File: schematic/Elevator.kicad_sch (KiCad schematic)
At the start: 25 parts, among them M1 Stepper_Motor_bipolar, Q1 Q_NMOS_GDS, Q2 Q_NMOS_GDS, Q3 Q_NMOS_GDS, SW1 SW_Push_LED, SW10 SW_Push_LED, SW11 SW_Push_LED, SW12 SW_Push_LED, SW13 SW_Push_LED, SW14 SW_Push_LED, SW15 SW_Push_LED, SW16 SW_Push_LED, SW2 SW_Push_LED, SW3 SW_Push_LED, SW4 SW_Push_LED, SW5 SW_Push_LED, SW6 SW_Push_LED, SW7 SW_Push_LED, SW8 SW_Push_LED, SW9 SW_Push_LED, U1 Pico, U2 74HC595, U3 74HC595

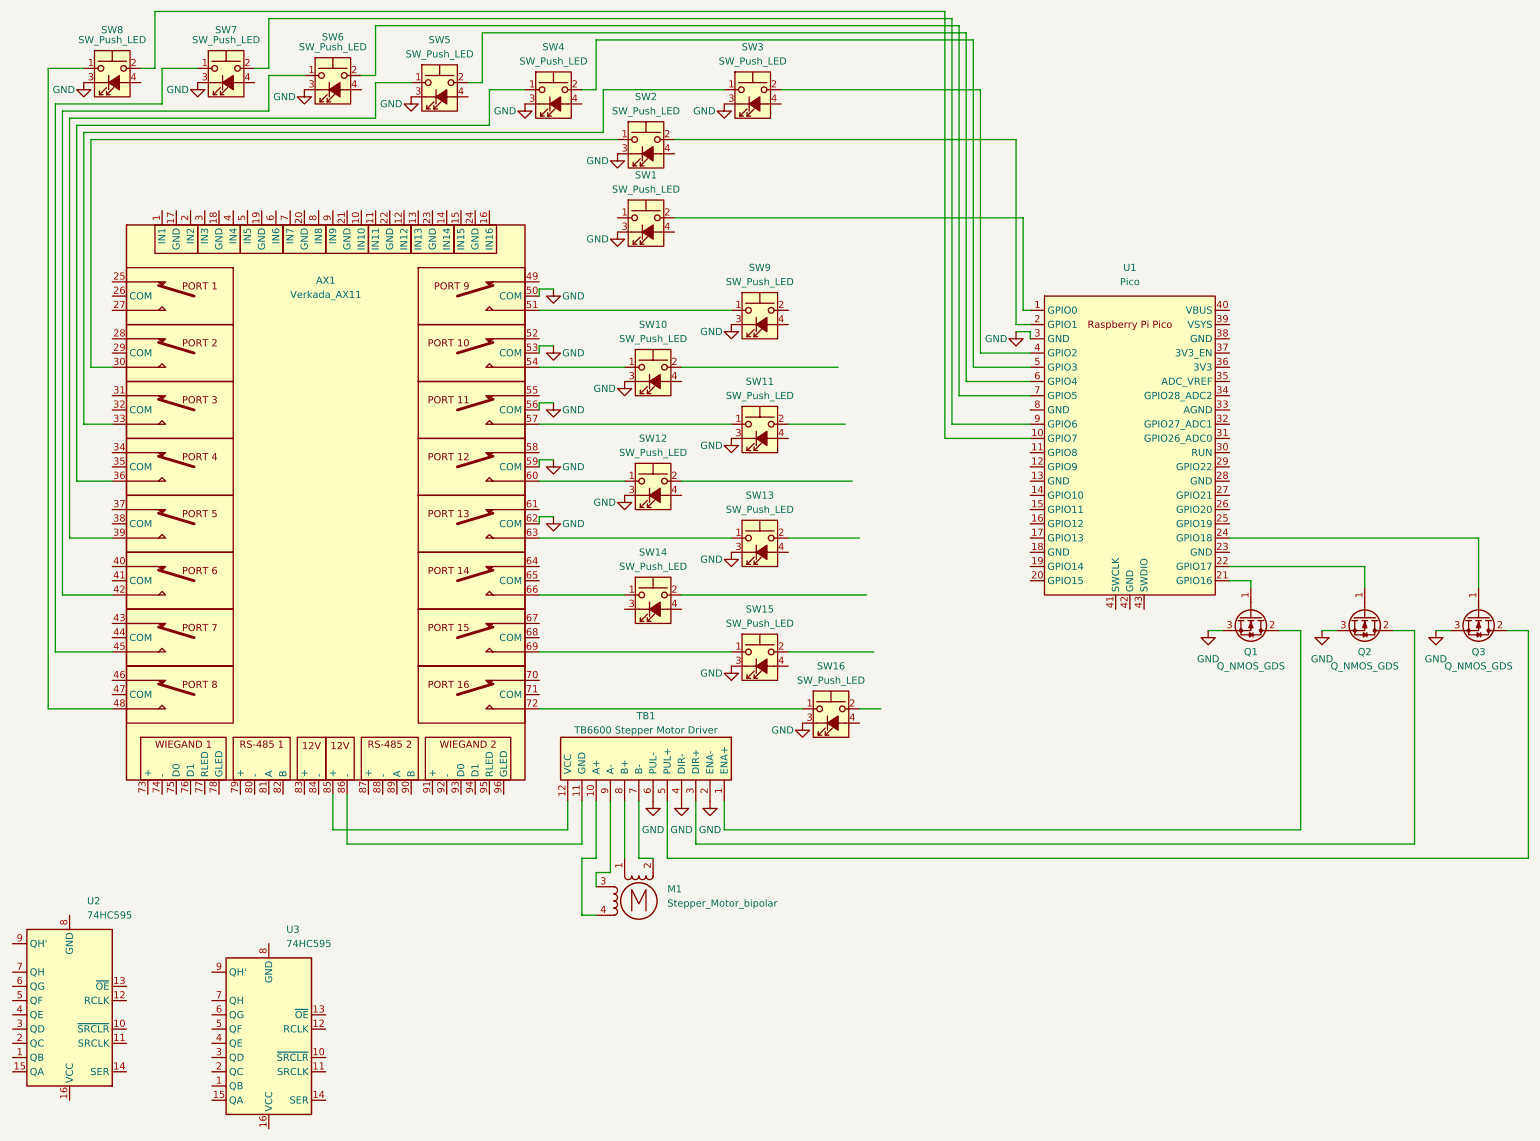
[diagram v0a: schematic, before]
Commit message: Kicad changes
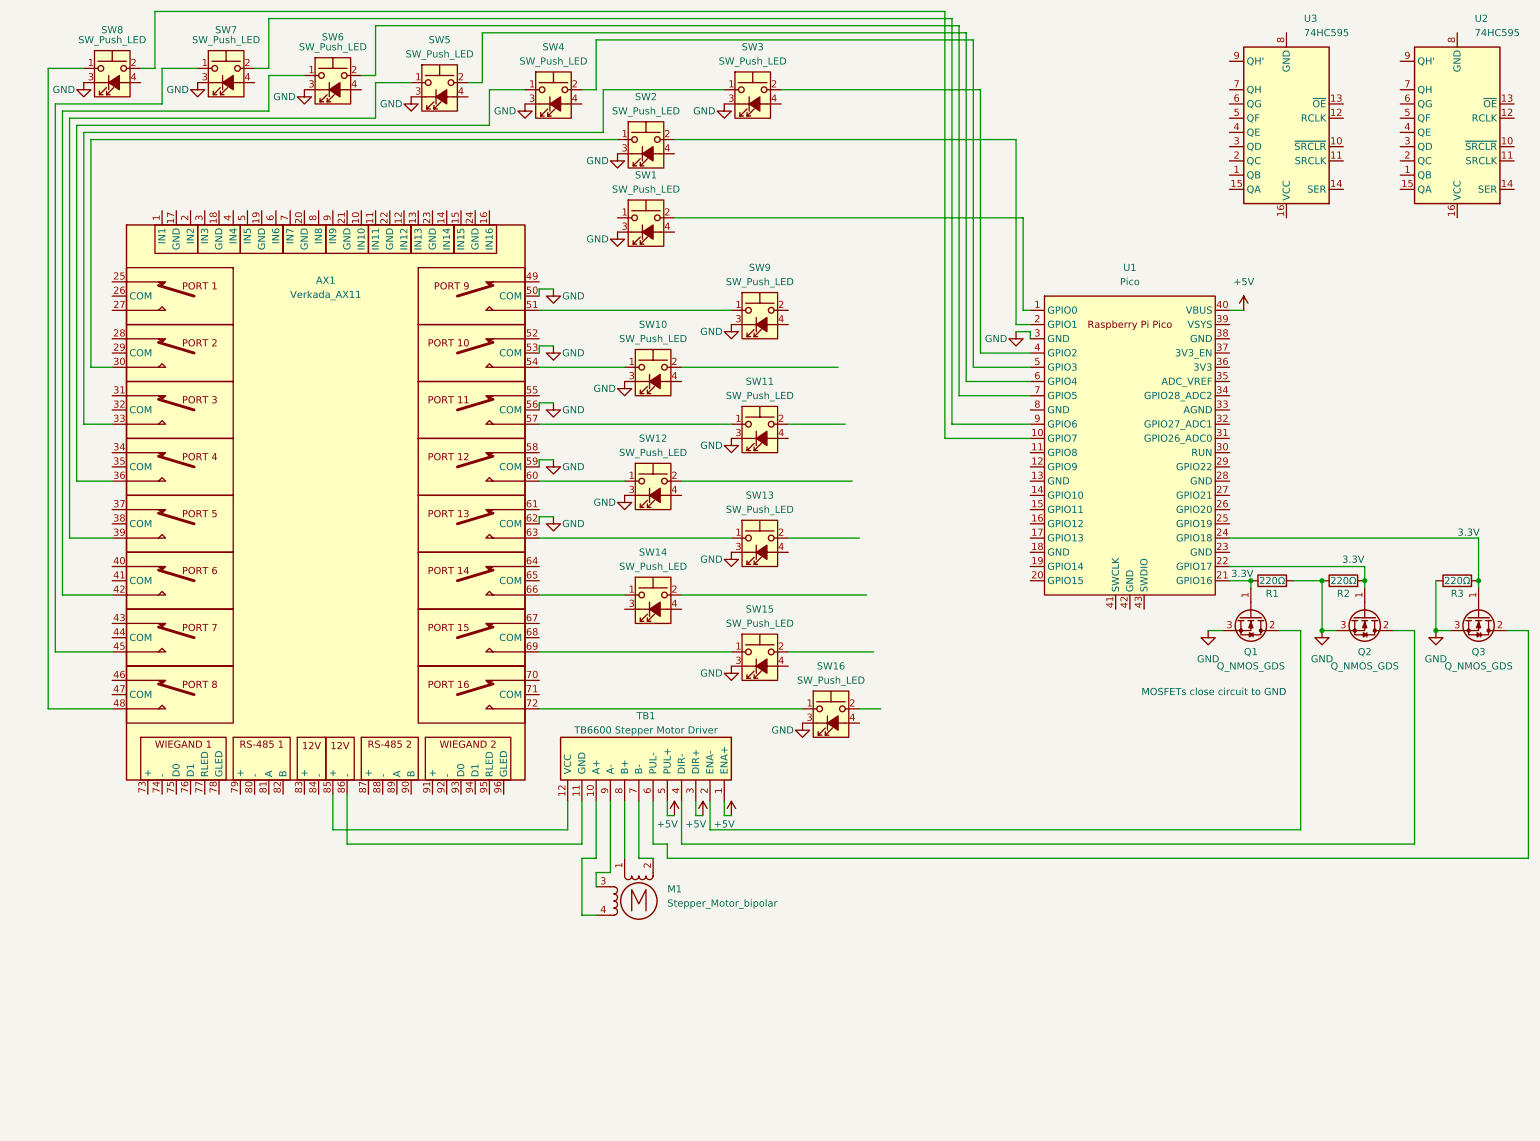
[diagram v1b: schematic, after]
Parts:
- added R1, R2, R3: 220Ω, symbol Device:R
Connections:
- net GND: now also R1.2, R2.1, R3.1; no longer TB1.2 (ENA-), TB1.4 (DIR-), TB1.6 (PUL-)
- net at Q2.1 (G), U1.22 (GPIO17): now also R2.2
- net at Q2.2 (D): now also TB1.4 (DIR-); no longer TB1.3 (DIR+)
- net at Q1.1 (G), U1.21 (GPIO16): now also R1.1
- net at Q3.1 (G), U1.24 (GPIO18): now also R3.2
- net +5V: now reaches U1.40 (VBUS)
- net +5V: now also TB1.1 (ENA+), TB1.3 (DIR+), TB1.5 (PUL+)
- net at Q1.2 (D): now also TB1.2 (ENA-); no longer TB1.1 (ENA+)
- net at Q3.2 (D): now also TB1.6 (PUL-); no longer TB1.5 (PUL+)
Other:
- note added: "3.3V"
- note added: "MOSFETs close circuit to GND"
- moved on the sheet: U2, U3
